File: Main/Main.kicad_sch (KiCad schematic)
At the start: 95 parts, among them J1 USB_B_Micro, J2 XT60, J3 Conn_01x03, J4 Conn_01x03, J5 Conn_01x03, J6 Conn_01x03, J7 MSD-4-A, Q2 Si2301CDS, SW1 SW_Push, SW2 SW_Push, U1 RP2350A-QFN60, U10 LM75B, U11 MCS1802GS-50-Z, U12 MCS1802GS-50-Z, U13 MCS1802GS-50-Z, U15 AP62150WU, U2 W25Q128JVS, U3 AMS1117-3.3, U4 MMC5983MA, U5 ICM-42688-P, U6 INA226, U7 KX134-1211, U8 MS5611-01BA, U9 MCS1802GS-50-Z, Y1 ABM8-272-T3

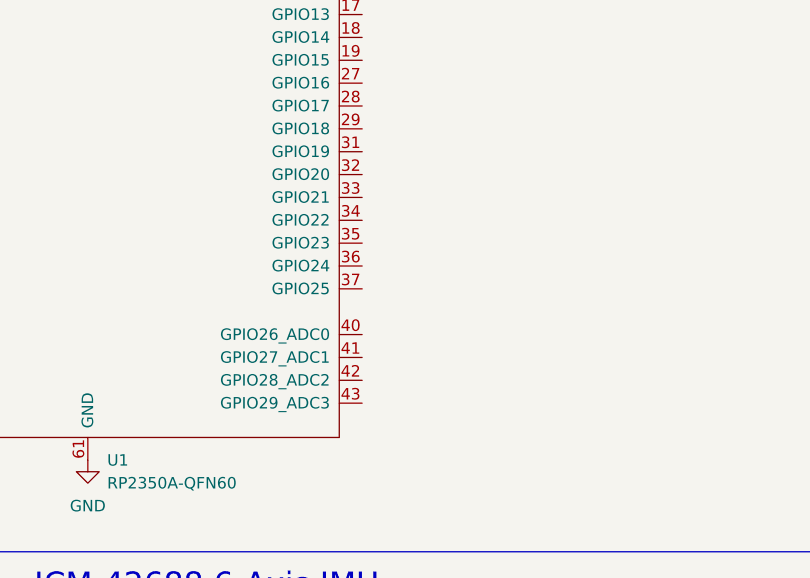
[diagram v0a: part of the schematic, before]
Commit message: more layout updates
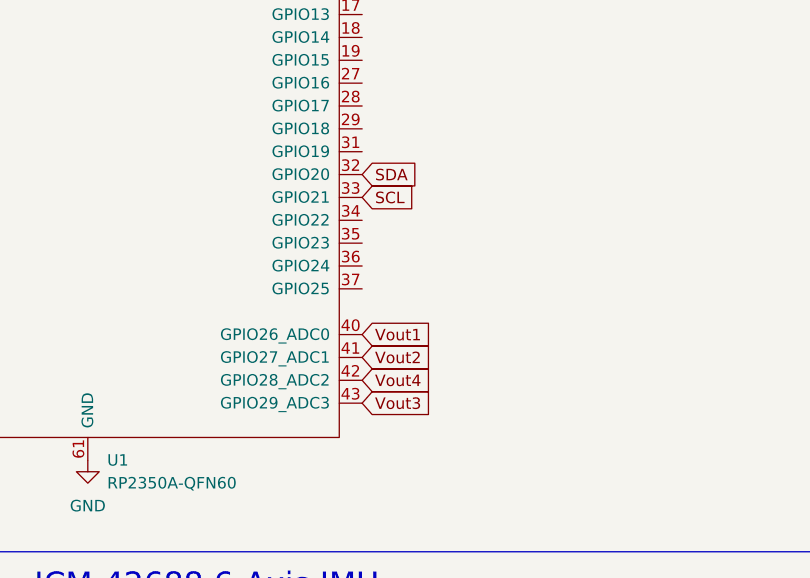
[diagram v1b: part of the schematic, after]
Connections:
- net SCL: now also U1.33 (GPIO21)
- net SDA: now also U1.32 (GPIO20)
- net Vout1: now also U1.40 (GPIO26_ADC0)
- net Vout2: now also U1.41 (GPIO27_ADC1)
- net Vout3: now also U1.43 (GPIO29_ADC3)
- net Vout4: now also U1.42 (GPIO28_ADC2)
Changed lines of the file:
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@@
+		)
+	)
+	(global_label "Vout1"
+		(shape input)
+		(at 212.09 143.51 0)
+		(fields_autoplaced yes)
+		(effects
+			(font
+				(size 1.27 1.27)
+			)
+			(justify left)
+		)
+		(property "Intersheetrefs" "${INTERSHEET_REFS}"
+			(at 220.397 143.51 0)
+			(effects
+				(font
+					(size 1.27 1.27)
+				)
+				(justify left)
+				(hide yes)
+			)
 		)
 	)
@@
 		)
 	)
+	(global_label "Vout4"
+		(shape input)
+		(at 212.09 148.59 0)
+		(fields_autoplaced yes)
+		(effects
+			(font
+				(size 1.27 1.27)
+			)
+			(justify left)
+		)
+		(property "Intersheetrefs" "${INTERSHEET_REFS}"
+			(at 220.397 148.59 0)
+			(effects
+				(font
+					(size 1.27 1.27)
+				)
+				(justify left)
+				(hide yes)
+			)
+		)
+	)
 	(global_label "SPI_SDI"
 		(shape input)
@@
 		)
 	)
+	(global_label "SDA"
+		(shape input)
+		(at 212.09 125.73 0)
+		(fields_autoplaced yes)
+		(effects
+			(font
+				(size 1.27 1.27)
+			)
+			(justify left)
+		)
+		(property "Intersheetrefs" "${INTERSHEET_REFS}"
+			(at 218.6433 125.73 0)
+			(effects
+				(font
+					(size 1.27 1.27)
+				)
+				(justify left)
+				(hide yes)
+			)
+		)
+	)
 	(global_label "current -1"
 		(shape input)
@@
 		)
 	)
+	(global_label "Vout3"
+		(shape input)
+		(at 212.09 151.13 0)
+		(fields_autoplaced yes)
+		(effects
+			(font
+				(size 1.27 1.27)
+			)
+			(justify left)
+		)
+		(property "Intersheetrefs" "${INTERSHEET_REFS}"
+			(at 220.397 151.13 0)
+			(effects
+				(font
+					(size 1.27 1.27)
+				)
+				(justify left)
+				(hide yes)
+			)
+		)
+	)
 	(global_label "SPI_SDI2"
 		(shape input)
@@
 				)
 				(justify right)
+				(hide yes)
+			)
+		)
+	)
+	(global_label "Vout2"
+		(shape input)
+		(at 212.09 146.05 0)
+		(fields_autoplaced yes)
+		(effects
+			(font
+				(size 1.27 1.27)
+			)
+			(justify left)
+		)
+		(property "Intersheetrefs" "${INTERSHEET_REFS}"
+			(at 220.397 146.05 0)
+			(effects
+				(font
+					(size 1.27 1.27)
+				)
+				(justify left)
 				(hide yes)
 			)
@@
 			(effects
 				(font
+					(size 1.27 1.27)
+				)
+				(justify left)
+				(hide yes)
+			)
+		)
+	)
+	(global_label "SCL"
+		(shape input)
+		(at 212.09 128.27 0)
+		(fields_autoplaced yes)
+		(effects
+			(font
+				(size 1.27 1.27)
+			)
+			(justify left)
+		)
+		(property "Intersheetrefs" "${INTERSHEET_REFS}"
+			(at 218.5828 128.27 0)
+			(effects
+				(font
